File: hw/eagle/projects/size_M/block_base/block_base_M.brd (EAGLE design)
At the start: 21 x 21 mm, 6 parts, among them IC1 ATTINY412-SSN

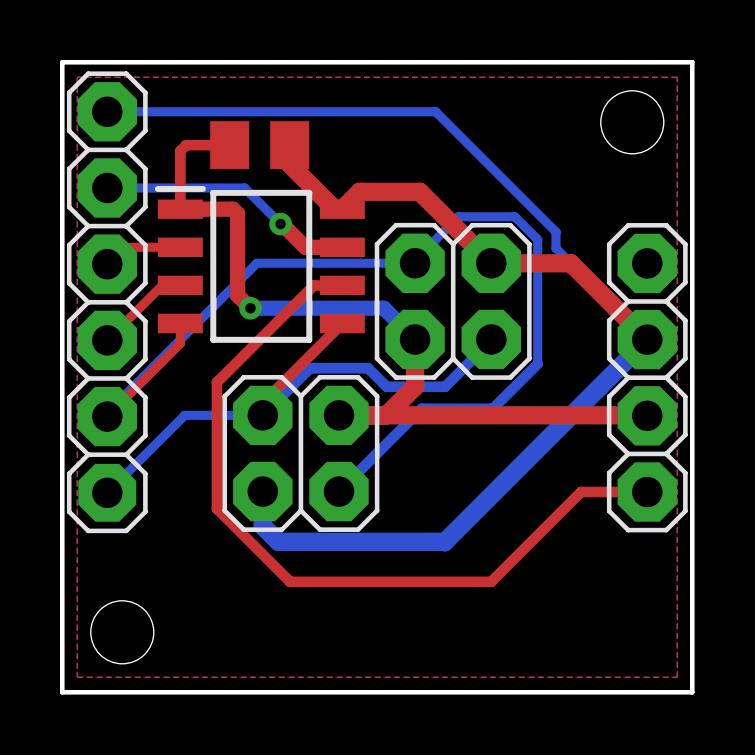
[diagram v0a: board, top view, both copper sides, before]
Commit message: completed pcb design for M.0 - made PCB order
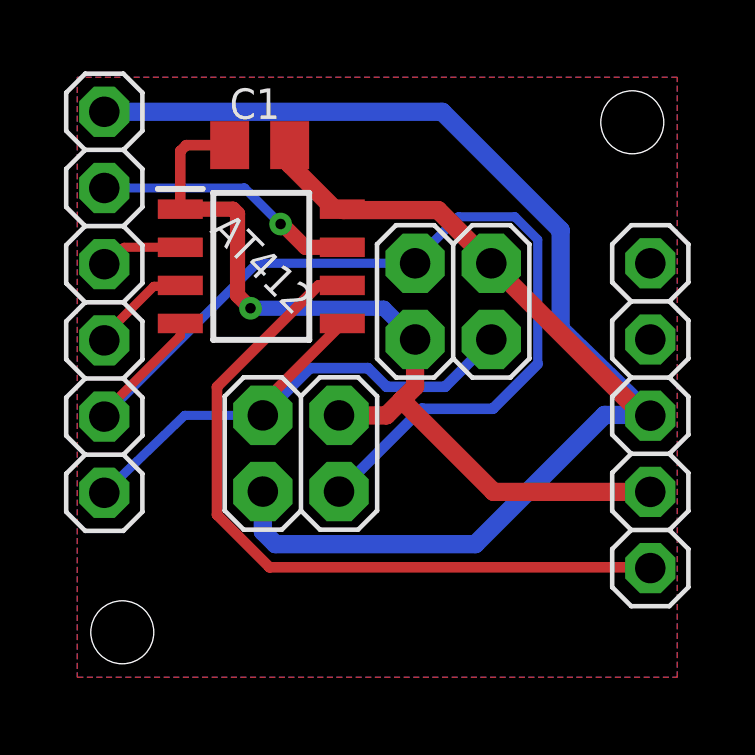
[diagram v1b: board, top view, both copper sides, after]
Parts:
- removed JP1: (no value), pinhead2:1X04
- added JP5: (no value), pinhead2:1X05
- AT412: value ATTINY412-SSN -> AT412
- moved JP2 0.10 mm to (1.40, 13.0)
- renumbered IC1 to AT412
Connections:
- net GND: now also JP5.3; no longer JP1.2
- net UPDI: now also JP5.5; no longer JP1.4
- net VDD: now also JP5.4; no longer JP1.3
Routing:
- net GND: track 54.0 -> 56.7 mm
- net UPDI: track 26.3 -> 25.0 mm
- net VDD: track 29.7 -> 28.9 mm
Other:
- board outline removed
- board text added: "VBAT"
- board text added: "VUSB"

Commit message: changes in pcb desingm - not finished and another minor changes in the documentation
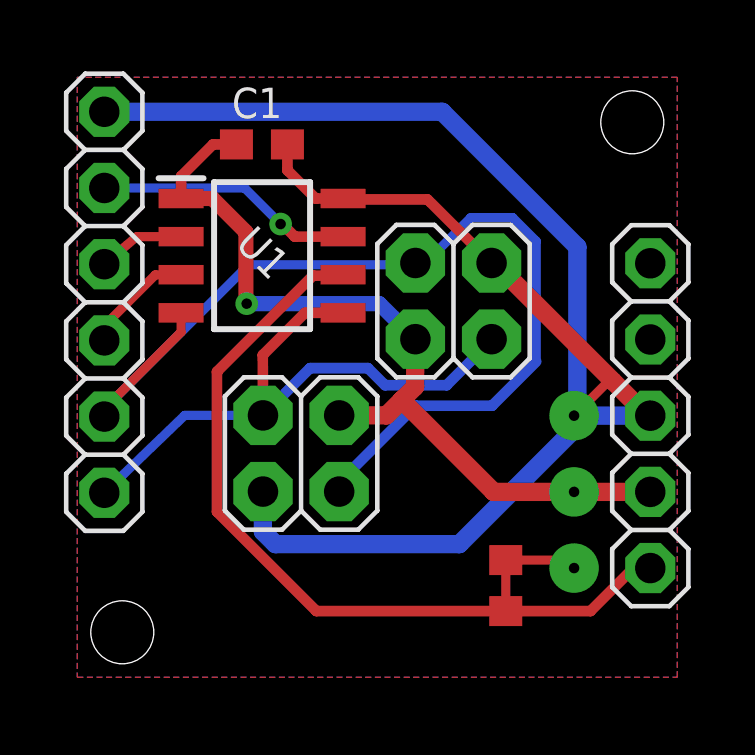
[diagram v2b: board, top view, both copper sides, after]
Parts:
- removed AT412: AT412, ATTINY412-SSN:SOIC127P600X175-8N
- removed JP3, JP4: (no value), pinhead2:2X02
- added J3, J4: (no value), pinhead2:2X02
- added R1: 4k7, rcl:R0603
- added U1: AT412, ATTINY412-SSN:SOIC127P600X175-8N
- C1: device rcl:C0805K -> rcl:C0603
- moved C1 0.08 mm to (6.65, 18.3)
- renumbered JP2 to J2, JP5 to J5
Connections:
- net GND: now also J3.4, J4.1, U1.8; no longer AT412.8, JP3.4, JP4.1
- net PA3: now also U1.7; no longer AT412.7
- net PA6: now also U1.2; no longer AT412.2
- net PA7: now also U1.3; no longer AT412.3
- net SCL: now also J3.3, J4.2, U1.5; no longer AT412.5, JP3.3, JP4.2
- net SDA: now also J3.2, J4.3, U1.4; no longer AT412.4, JP3.2, JP4.3
- net UPDI: now also R1.1, R1.2, U1.6; no longer AT412.6
- net VDD: now also J3.1, J4.4, U1.1; no longer AT412.1, JP3.1, JP4.4
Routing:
- net UPDI: track 25.0 -> 30.7 mm, vias 0 -> 1
- net VDD: track 28.9 -> 30.8 mm, vias 1 -> 2
- net GND: track 56.7 -> 58.2 mm, vias 0 -> 1
- net SCL: track 19.8 -> 20.9 mm
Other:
- board text added: "base M.1"
- board text removed: "base M.0"
